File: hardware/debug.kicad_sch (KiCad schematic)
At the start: 32 parts, among them U19 74HC04, U20 74HC540, U21 74HC541, U22 74HC541, U23 74HC541, U24 74HC541

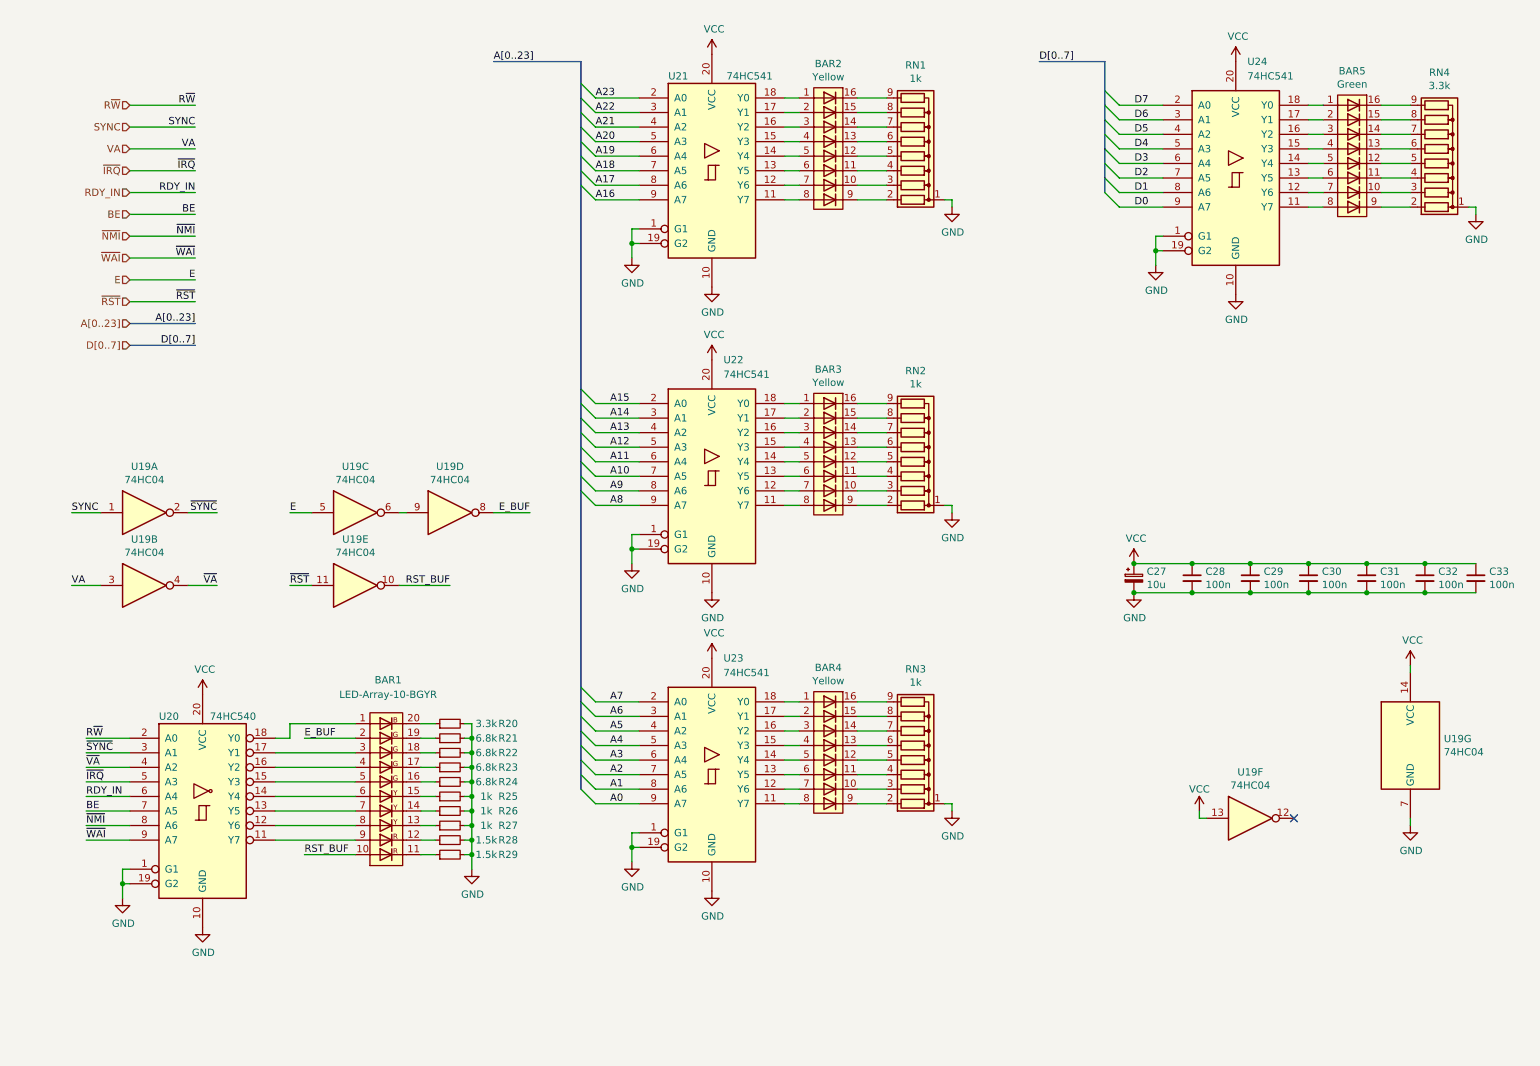
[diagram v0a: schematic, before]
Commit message: Update schematic
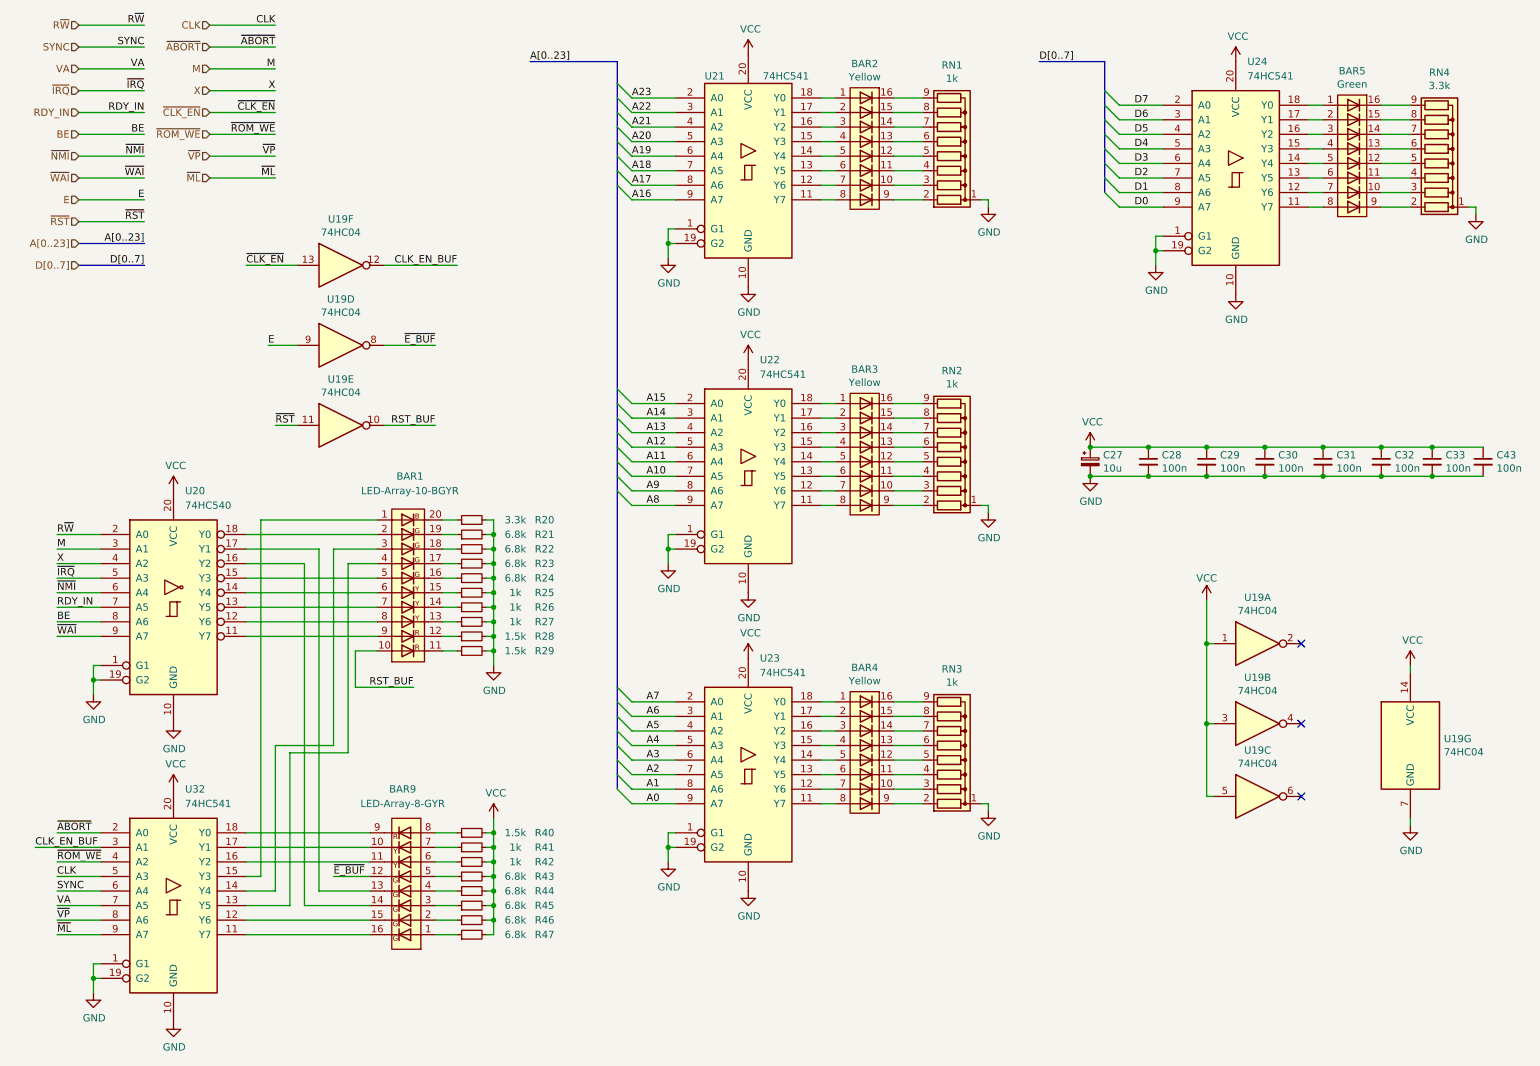
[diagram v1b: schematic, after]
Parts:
- added BAR9: LED-Array-8-GYR, symbol 65C816:LED-Array-8-GYR
- added C43: 100n, symbol Device:C_Small
- added R40: 1.5k, symbol Device:R_Small
- added R41, R42: 1k, symbol Device:R_Small
- added R43, R44, R45, R46, R47: 6.8k, symbol Device:R_Small
- added U32: 74HC541, symbol 74xx:74LS541
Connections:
- net BE: now also U20.8 (A6); no longer U20.7 (A5)
- net E: now also U19.9; no longer U19.5
- net GND: now also C43.2, U32.1 (G1), U32.10 (GND), U32.19 (G2)
- net RDY_IN: now also U20.7 (A5); no longer U20.6 (A4)
- net SYNC: now also U32.6 (A4); no longer U19.1
- net VA: now also U32.7 (A5); no longer U19.3
- net VCC: now also U19.1, U19.3, U19.5, C43.1, R40.2, R41.2, R42.2, R43.2, R44.2, R45.2, R46.2, R47.2, U32.20 (VCC); no longer U19.13
- net ~{NMI}: now also U20.6 (A4); no longer U20.8 (A6)
- net CLK_EN_BUF: now reaches U19.12
- net CLK_EN_BUF: now also U32.3 (A1)
- net at U19.6: no longer U19.9
- net at U20.16 (Y2): now also BAR9.14 (K); no longer BAR1.4 (A)
- net at U20.17 (Y1): now also BAR9.13 (K); no longer BAR1.3 (A)
- net at U20.18 (Y0): now also BAR1.2 (A); no longer BAR1.1 (A)
- net E_BUF renamed ~{E_BUF}
- net ~{E_BUF}: now also BAR9.12 (K); no longer BAR1.2 (A)
- net ~{SYNC}: no longer names the net of U19.2
- net ~{SYNC}: no longer U20.3 (A1)
- net ~{VA}: no longer names the net of U19.4
- net ~{VA}: no longer U20.4 (A2)
- new net: BAR9.1 (A), R47.1
- new net: BAR9.10 (K), U32.17 (Y1)
- new net: BAR9.11 (K), U32.16 (Y2)
- new net: BAR9.15 (K), U32.12 (Y6)
- new net: BAR9.16 (K), U32.11 (Y7)
- new net: BAR9.2 (A), R46.1
- new net: BAR9.3 (A), R45.1
- new net: BAR9.4 (A), R44.1
- new net: BAR9.5 (A), R43.1
- new net: BAR9.6 (A), R42.1
- new net: BAR9.7 (A), R41.1
- new net: BAR9.8 (A), R40.1
- new net: BAR9.9 (K), U32.18 (Y0)
- new net: BAR1.1 (A), U32.15 (Y3)
- new net: BAR1.3 (A), U32.14 (Y4)
- new net: BAR1.4 (A), U32.13 (Y5)
- new net CLK: U32.5 (A3)
- new net M: U20.3 (A1)
- new net X: U20.4 (A2)
- new net ~{ABORT}: U32.2 (A0)
- new net ~{CLK_EN}: U19.13
- new net ~{ML}: U32.9 (A7)
- new net ~{ROM_WE}: U32.4 (A2)
- new net ~{VP}: U32.8 (A6)
- no-connect marks 1 -> 3
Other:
- moved on the sheet: BAR1, BAR2, BAR3, BAR4, C27, C28, C29, C30, C31, C32, C33, R20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
